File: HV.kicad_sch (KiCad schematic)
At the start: 48 parts, among them J1 HVConnector, J2 ExportConnector, J3 PrechargeContactor, J4 PrechargeContactor, U1 TLV9002QDRQ1, U2 LT1963AEST-3.3#TRPBF, U3 TLV9002QDRQ1

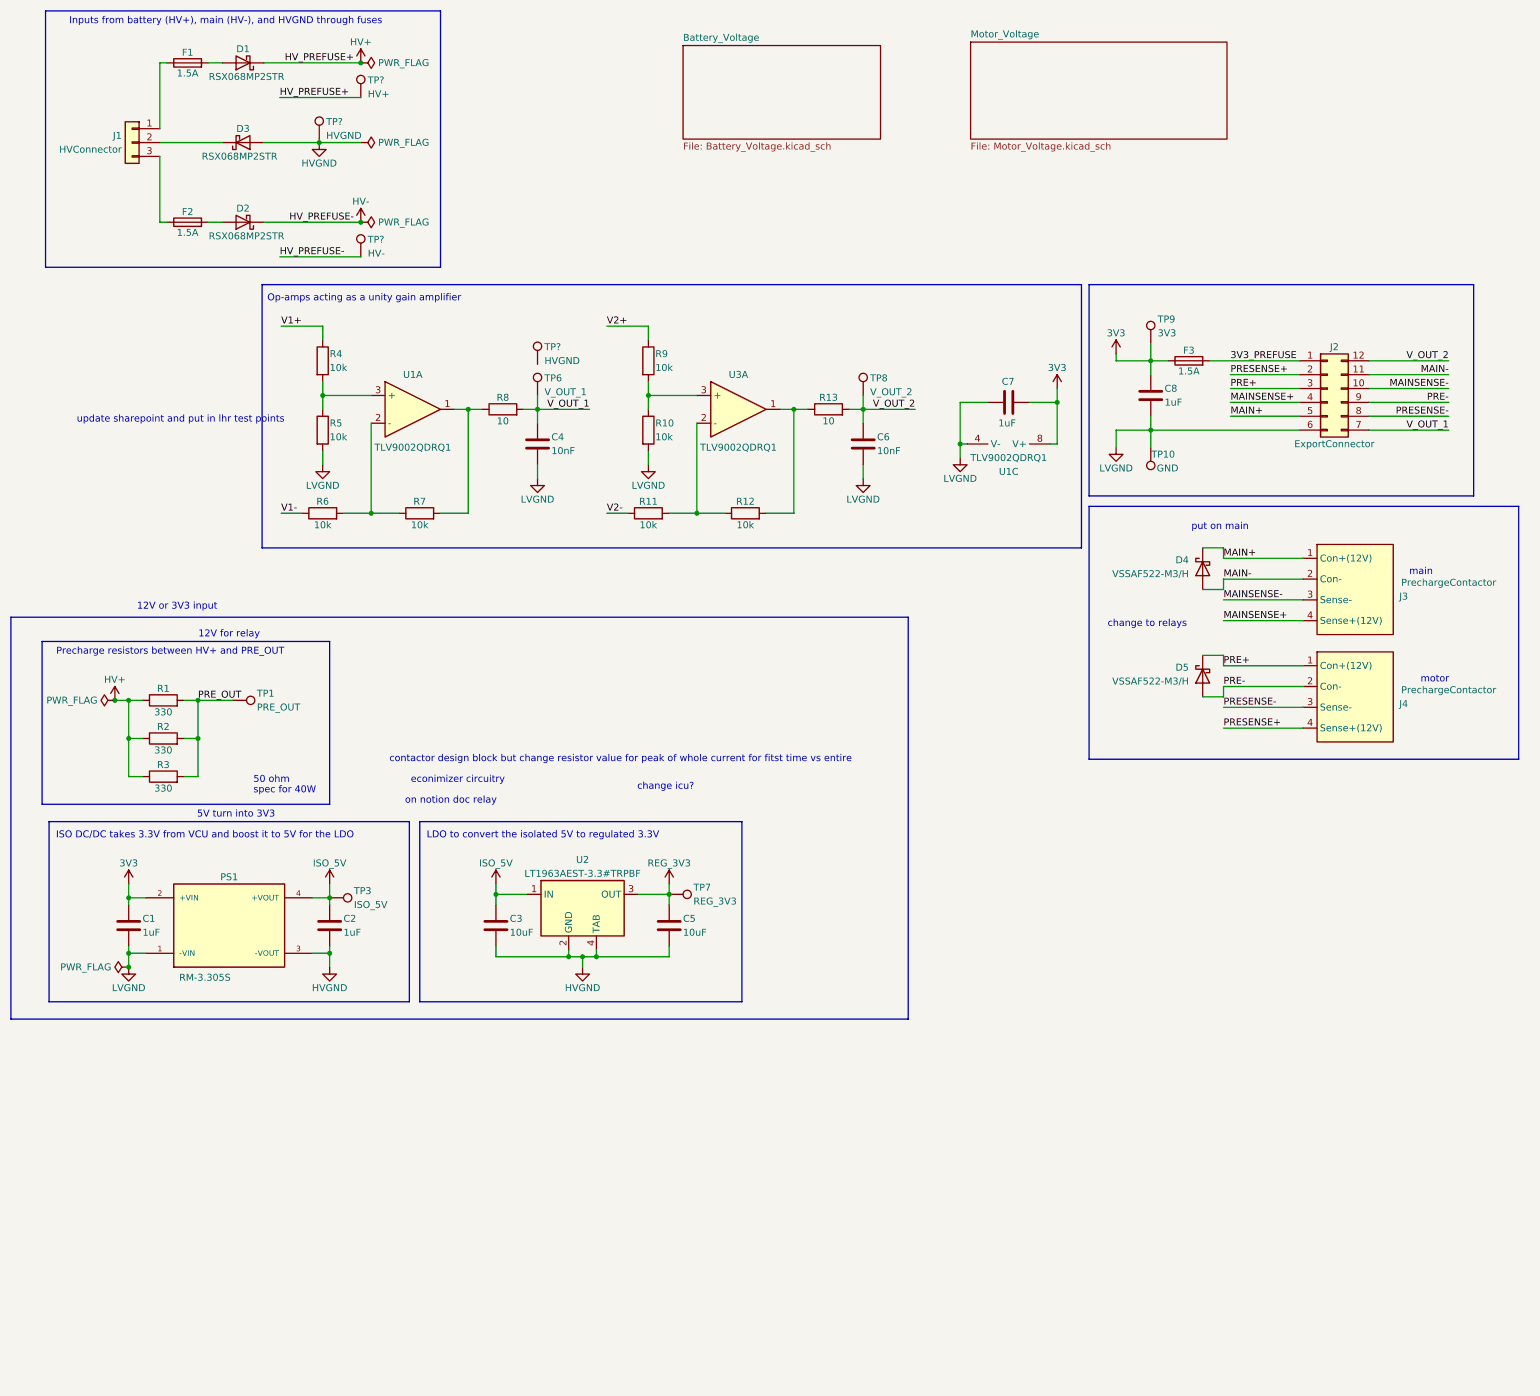
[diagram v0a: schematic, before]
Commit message: shifted hierarchical sheets
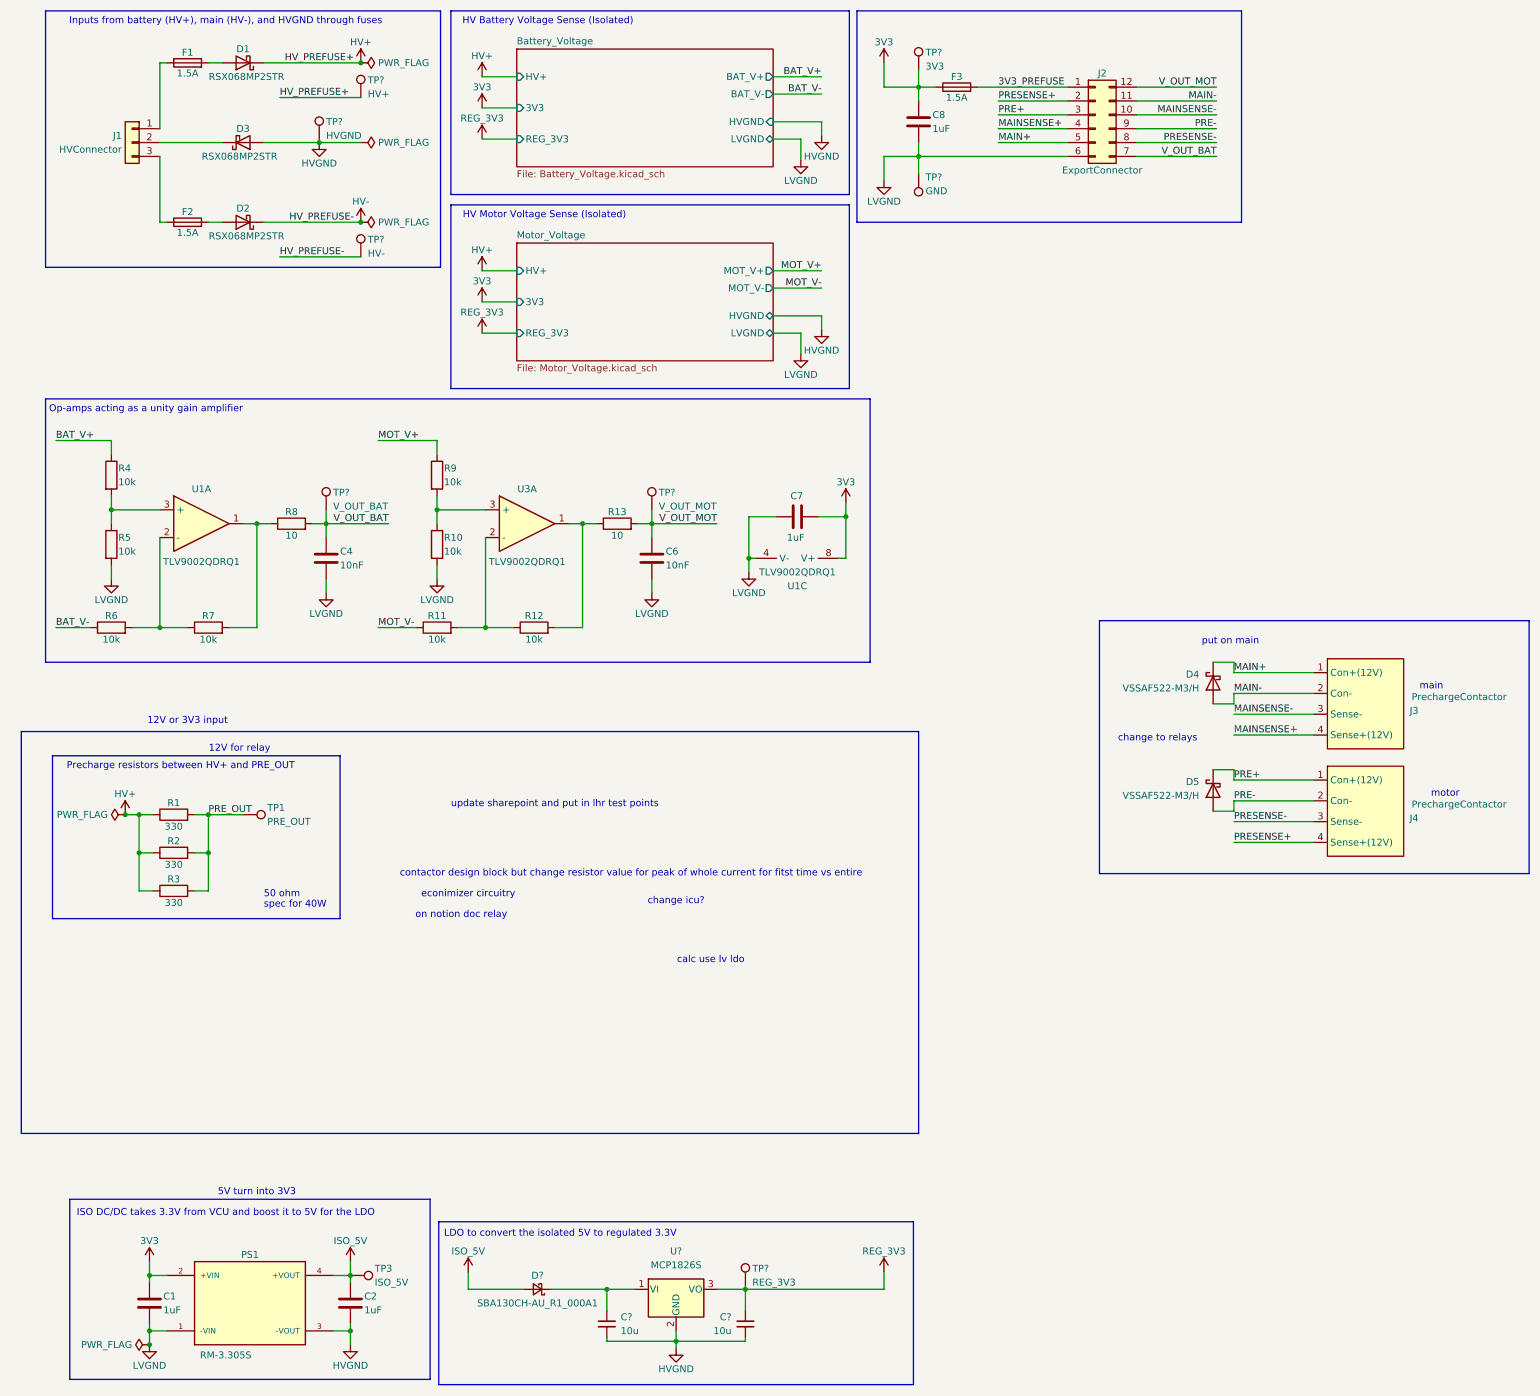
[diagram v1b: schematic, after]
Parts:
- removed C3, C5: 10uF, symbol Device:C
- removed TP10: GND, symbol Connector:TestPoint
- removed TP6: V_OUT_1, symbol Connector:TestPoint
- removed TP7: REG_3V3, symbol Connector:TestPoint
- removed TP8: V_OUT_2, symbol Connector:TestPoint
- removed TP9: 3V3, symbol Connector:TestPoint
- removed U2: LT1963AEST-3.3#TRPBF, ActivePrecharge-RevB:VREG_LT1963AEST-3.3_TRPBF, symbol Regulator_Linear:LT1963AxST-3.3
- added C? (x2): 10u, Capacitor_SMD:C_0805_2012Metric_Pad1.18x1.45mm_HandSolder, symbol Device:C_Small
- added D?: SBA130CH-AU_R1_000A1, Diode_SMD:D_SOD-323_HandSoldering, symbol Device:D_Schottky_Small
- added TP?: V_OUT_MOT, TestPoint:TestPoint_Loop_D1.80mm_Drill1.0mm_Beaded, symbol lhrs_misc:Multimeter_TP
- added TP?: 3V3, TestPoint:TestPoint_Loop_D1.80mm_Drill1.0mm_Beaded, symbol lhrs_misc:Multimeter_TP
- added TP?: REG_3V3, TestPoint:TestPoint_Loop_D1.80mm_Drill1.0mm_Beaded, symbol lhrs_misc:Multimeter_TP
- added TP?: GND, TestPoint:TestPoint_Loop_D1.80mm_Drill1.0mm_Beaded, symbol lhrs_misc:Multimeter_TP
- added U?: MCP1826S, Package_TO_SOT_SMD:SOT-223-3_TabPin2, symbol Regulator_Linear:MCP1826S
- TP?: value HVGND -> V_OUT_BAT
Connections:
- net V_OUT_1 is gone; now on net V_OUT_BAT: C4.1, J2.7 (Pin_7), R8.2
- net 3V3: now also TP?.1
- net HVGND: now also C?.1, C?.1, U?.2 (GND)
- net ISO_5V: now also D?.2 (A)
- net LVGND: now also TP?.1
- net REG_3V3: now also C?.2, TP?.1, U?.3 (VO)
- net V_OUT_BAT: now reaches TP?.1
- net V1+ renamed BAT_V+
- net V1- renamed BAT_V-
- net V2+ renamed MOT_V+
- net V2- renamed MOT_V-
- net V_OUT_2 renamed V_OUT_MOT
- net V_OUT_MOT: now also TP?.1
- new net: C?.2, D?.1 (K), U?.1 (VI)
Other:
- sheet Battery_Voltage ports: added 3V3, BAT_V+, BAT_V-, HV+, HVGND, LVGND, REG_3V3; removed none
- sheet Motor_Voltage ports: added 3V3, HV+, HVGND, LVGND, MOT_V+, MOT_V-, REG_3V3; removed none
- note added: "HV Battery Voltage Sense (Isolated)"
- note added: "HV Motor Voltage Sense (Isolated)"
- note added: "calc use lv ldo"
- moved on the sheet: C1, C2, C4, C6, C7, C8, D4, D5, F3, J2, J3, J4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
